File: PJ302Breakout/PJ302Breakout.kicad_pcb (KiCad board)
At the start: 2 copper layers, 12.7 x 21.1 mm, 3 parts, among them J1 PJ302M, J2 Conn_01x04, J3 Conn_01x02

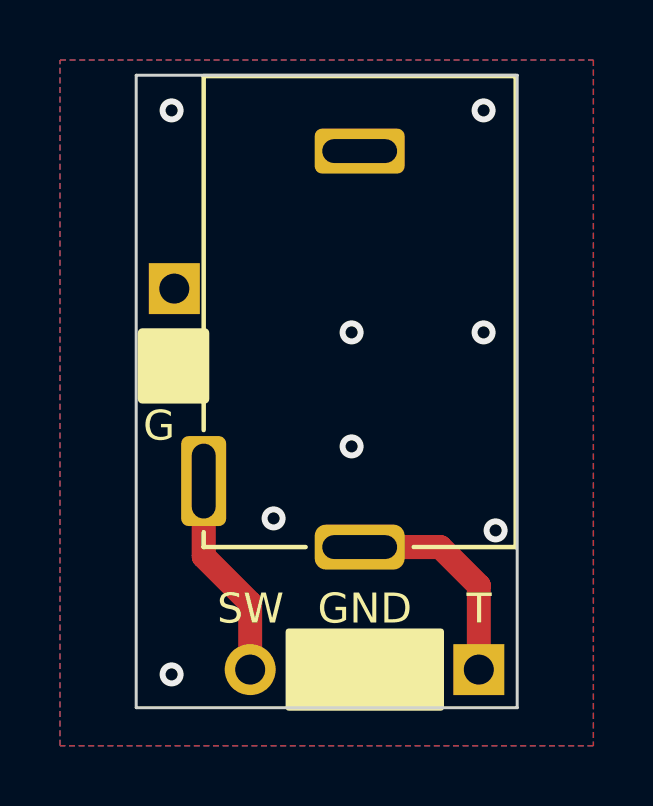
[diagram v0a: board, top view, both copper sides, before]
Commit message: PJ302 for BB
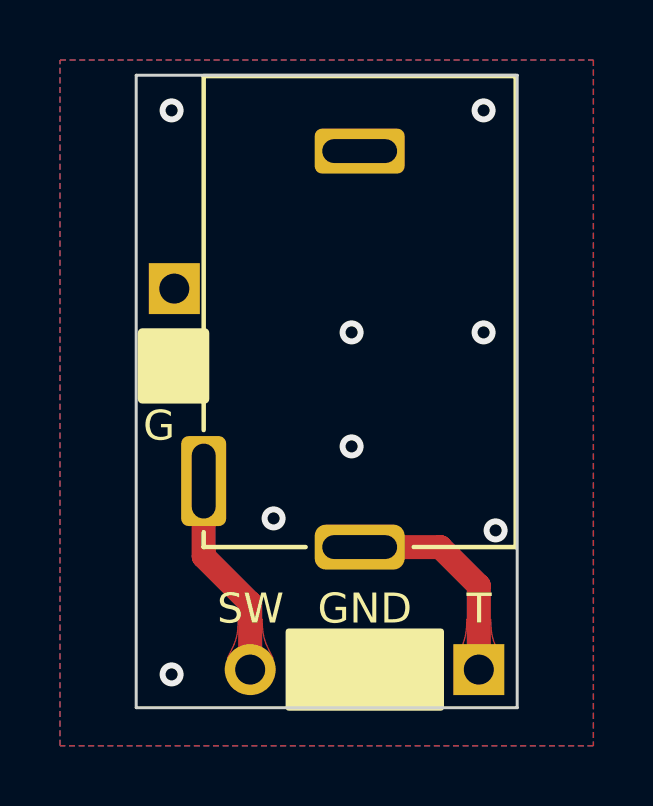
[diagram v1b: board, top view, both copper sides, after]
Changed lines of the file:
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@@
   (segment (start 116.6695 61.956) (end 119.356 61.956) (width 0.8) (layer "F.Cu") (net 3))
   (segment (start 120.64 63.24) (end 120.64 66.04) (width 0.8) (layer "F.Cu") (net 3))
+  (zone (net 2) (net_name "/sw") (layer "F.Cu") (hatch edge 0.508)
+    (priority 16962)
+    (connect_pads yes (clearance 0))
+    (min_thickness 0.0254) (filled_areas_thickness no)
+    (fill yes (thermal_gap 0.508) (thermal_bridge_width 0.508))
+    (polygon
+      (pts
+        (xy 112.62 64.35)
+        (xy 112.616314 64.539793)
+        (xy 112.605273 64.702112)
+        (xy 112.586901 64.842441)
+        (xy 112.56122 64.966261)
+        (xy 112.528256 65.079054)
+        (xy 112.488031 65.186303)
+        (xy 112.440569 65.293489)
+        (xy 112.385894 65.406095)
+        (xy 112.32403 65.529602)
+        (xy 112.255 65.669494)
+        (xy 113.02 66.465)
+        (xy 113.785 65.669494)
+        (xy 113.715969 65.529602)
+        (xy 113.654105 65.406095)
+        (xy 113.59943 65.293489)
+        (xy 113.551968 65.186303)
+        (xy 113.511743 65.079054)
+        (xy 113.478779 64.966261)
+        (xy 113.453098 64.842441)
+        (xy 113.434726 64.702112)
+        (xy 113.423685 64.539793)
+        (xy 113.42 64.35)
+      )
+    )
+  )
+  (zone (net 3) (net_name "Net-(J1-Pad3)") (layer "F.Cu") (hatch edge 0.508)
+    (priority 16962)
+    (connect_pads yes (clearance 0))
+    (min_thickness 0.0254) (filled_areas_thickness no)
+    (fill yes (thermal_gap 0.508) (thermal_bridge_width 0.508))
+    (polygon
+      (pts
+        (xy 120.24 64.35)
+        (xy 120.236314 64.539793)
+        (xy 120.225273 64.702112)
+        (xy 120.206901 64.842441)
+        (xy 120.18122 64.966261)
+        (xy 120.148256 65.079054)
+        (xy 120.108031 65.186303)
+        (xy 120.060569 65.293489)
+        (xy 120.005894 65.406095)
+        (xy 119.94403 65.529602)
+        (xy 119.875 65.669494)
+        (xy 120.64 66.465)
+        (xy 121.405 65.669494)
+        (xy 121.335969 65.529602)
+        (xy 121.274105 65.406095)
+        (xy 121.21943 65.293489)
+        (xy 121.171968 65.186303)
+        (xy 121.131743 65.079054)
+        (xy 121.098779 64.966261)
+        (xy 121.073098 64.842441)
+        (xy 121.054726 64.702112)
+        (xy 121.043685 64.539793)
+        (xy 121.04 64.35)
+      )
+    )
+  )
   (zone (net 1) (net_name "GND") (layers F&B.Cu) (hatch edge 0.508)
     (connect_pads (clearance 0.508))
@@
       )
     )
+  )
+  (zone (net 3) (net_name "Net-(J1-Pad3)") (layer "F.Cu") (hatch edge 0.508)
+    (priority 16962)
+    (connect_pads yes (clearance 0))
+    (min_thickness 0.0254) (filled_areas_thickness no)
+    (fill yes (thermal_gap 0.508) (thermal_bridge_width 0.508))
+    (polygon
+      (pts
+        (xy 118.1595 61.556)
+        (xy 117.993132 61.553825)
+        (xy 117.849637 61.547047)
+        (xy 117.724609 61.53528)
+        (xy 117.613642 61.518142)
+        (xy 117.512331 61.495247)
+        (xy 117.416271 61.466213)
+        (xy 117.321055 61.430655)
+        (xy 117.222277 61.388189)
+        (xy 117.115533 61.338432)
+        (xy 116.996417 61.281)
+        (xy 116.2945 61.956)
+        (xy 116.996417 62.631)
+        (xy 117.115533 62.573567)
+        (xy 117.222277 62.52381)
+        (xy 117.321055 62.481344)
+        (xy 117.416271 62.445786)
+        (xy 117.512331 62.416752)
+        (xy 117.613642 62.393857)
+        (xy 117.724609 62.376719)
+        (xy 117.849637 62.364952)
+        (xy 117.993132 62.358174)
+        (xy 118.1595 62.356)
+      )
+    )
+  )
+  (zone (net 2) (net_name "/sw") (layer "F.Cu") (hatch edge 0.508)
+    (priority 16962)
+    (connect_pads yes (clearance 0))
+    (min_thickness 0.0254) (filled_areas_thickness no)
+    (fill yes (thermal_gap 0.508) (thermal_bridge_width 0.508))
+    (polygon
+      (pts
+        (xy 111.8695 61.246)
+        (xy 111.871674 61.079632)
+        (xy 111.878452 60.936137)
+        (xy 111.890219 60.811109)
+        (xy 111.907357 60.700142)
+        (xy 111.930252 60.598831)
+        (xy 111.959286 60.502771)
+        (xy 111.994844 60.407555)
+        (xy 112.03731 60.308777)
+        (xy 112.087067 60.202033)
+        (xy 112.1445 60.082917)
+        (xy 111.4695 59.381)
+        (xy 110.7945 60.082917)
+        (xy 110.851932 60.202033)
+        (xy 110.901689 60.308777)
+        (xy 110.944155 60.407555)
+        (xy 110.979713 60.502771)
+        (xy 111.008747 60.598831)
+        (xy 111.031642 60.700142)
+        (xy 111.04878 60.811109)
+        (xy 111.060547 60.936137)
+        (xy 111.067325 61.079632)
+        (xy 111.0695 61.246)
+      )
+    )
